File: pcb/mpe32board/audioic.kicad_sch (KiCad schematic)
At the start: 13 parts, among them J47 AudioJack3_Ground, U1 TAC5212IRGER

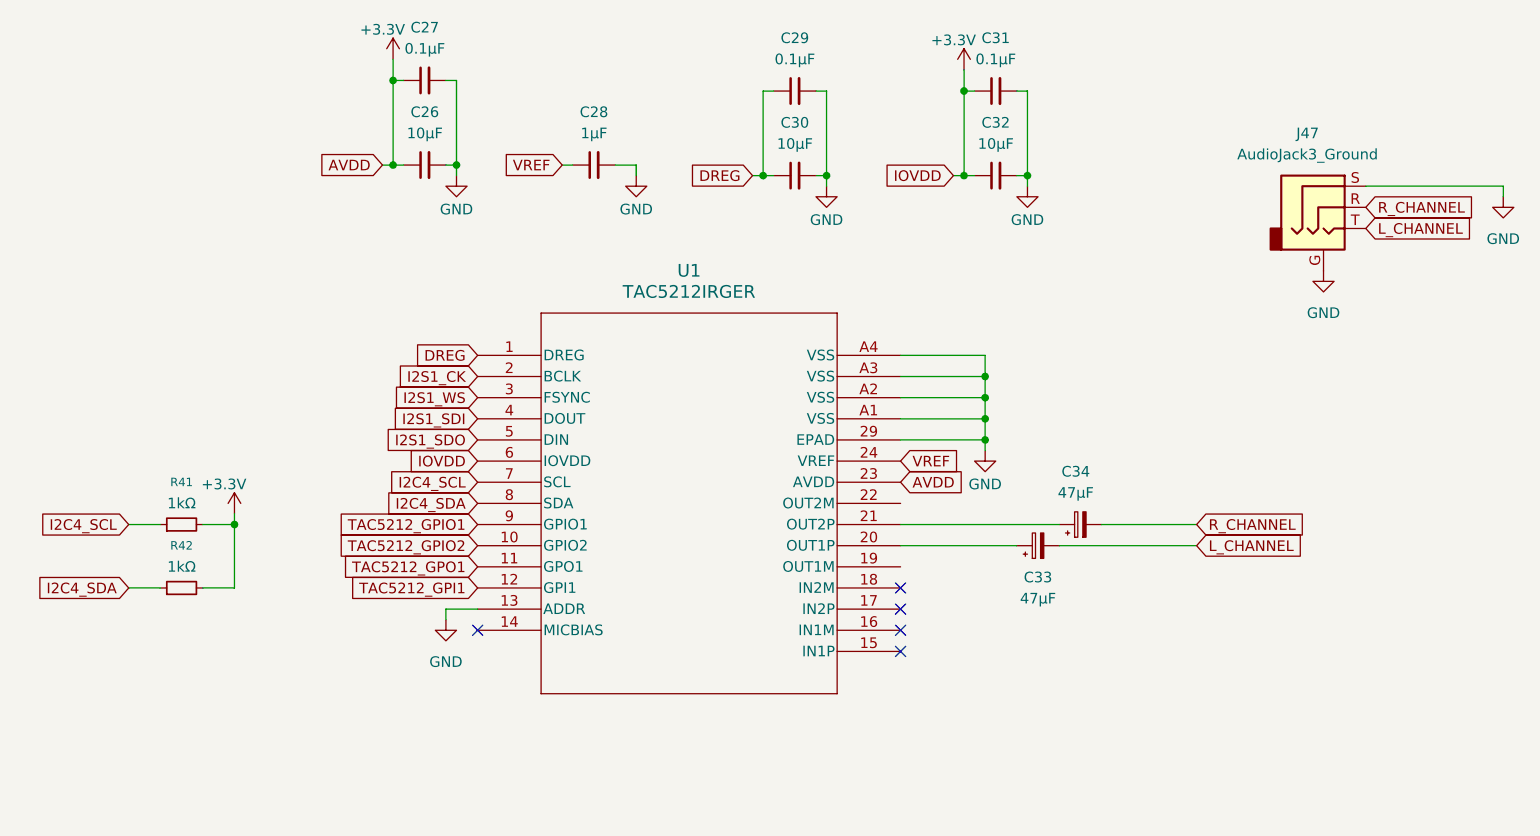
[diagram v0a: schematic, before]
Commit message: layout stuff
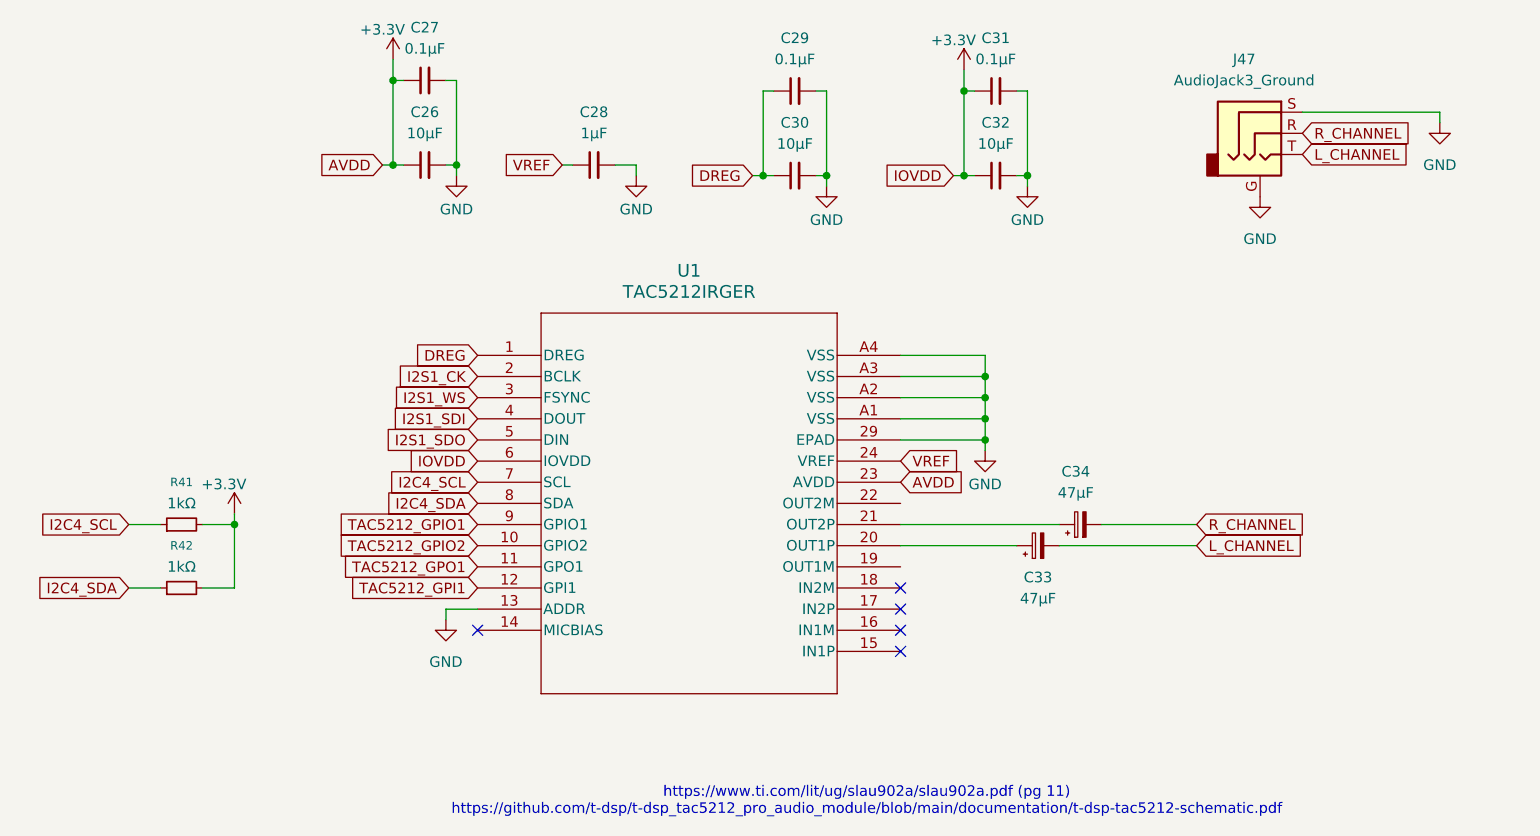
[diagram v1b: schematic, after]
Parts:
- C26, C27, C28, C29, C30, C31, C32, C33, C34: footprint (none) -> Capacitor_SMD:C_0603_1608Metric
- R41, R42: footprint (none) -> Resistor_SMD:R_0603_1608Metric
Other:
- note added: "https://www.ti.com/lit/ug/slau902a/slau902a.pdf (pg 11) https://github.com/t-dsp/t-dsp_tac5212_pro_audio_module/blob/main/documentation/t-dsp-tac5212-schematic.pdf"
- moved on the sheet: J47
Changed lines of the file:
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@@
 	(generator_version "9.0")
 	(paper "A4")
+	(text "https://www.ti.com/lit/ug/slau902a/slau902a.pdf (pg 11)\nhttps://github.com/t-dsp/t-dsp_tac5212_pro_audio_module/blob/main/documentation/t-dsp-tac5212-schematic.pdf"
+		(exclude_from_sim no)
+		(at 176.276 133.604 0)
+		(effects
+			(font
+				(size 1.27 1.27)
+			)
+		)
+	)
 	(junction
 		(at 119.38 57.15)
@@
 	(wire
 		(pts
-			(xy 252.73 60.96) (xy 252.73 59.69)
+			(xy 245.11 52.07) (xy 245.11 50.8)
 		)
 		(stroke
@@
 	(wire
 		(pts
-			(xy 252.73 59.69) (xy 236.22 59.69)
+			(xy 245.11 50.8) (xy 228.6 50.8)
 		)
 		(stroke
@@
 	(global_label "L_CHANNEL"
 		(shape input)
-		(at 236.22 64.77 0)
+		(at 228.6 55.88 0)
 		(fields_autoplaced yes)
 		(effects
@@
 		)
 		(property "Intersheetrefs" "${INTERSHEET_REFS}"
-			(at 249.7281 64.77 0)
+			(at 242.1081 55.88 0)
 			(effects
 				(font
@@
 	(global_label "R_CHANNEL"
 		(shape input)
-		(at 236.22 62.23 0)
+		(at 228.6 53.34 0)
 		(fields_autoplaced yes)
 		(effects
@@
 		)
 		(property "Intersheetrefs" "${INTERSHEET_REFS}"
-			(at 249.97 62.23 0)
+			(at 242.35 53.34 0)
 			(effects
 				(font
@@
 			)
 		)
-		(property "Footprint" ""
+		(property "Footprint" "Capacitor_SMD:C_0603_1608Metric"
 			(at 191.77 58.42 0)
 			(effects
@@
 			)
 		)
-		(property "Footprint" ""
+		(property "Footprint" "Capacitor_SMD:C_0603_1608Metric"
 			(at 167.64 48.26 0)
 			(effects
@@
 	(symbol
 		(lib_id "power:GND")
-		(at 231.14 69.85 0)
+		(at 223.52 60.96 0)
 		(unit 1)
 		(exclude_from_sim no)
@@
 		(fields_autoplaced yes)
 		(property "Reference" "#PWR0150"
-			(at 231.14 76.2 0)
+			(at 223.52 67.31 0)
 			(effects
 				(font
@@
 		)
 		(property "Value" "GND"
-			(at 231.14 74.93 0)
+			(at 223.52 66.04 0)
 			(effects
 				(font
@@
 		)
 		(property "Footprint" ""
-			(at 231.14 69.85 0)
+			(at 223.52 60.96 0)
 			(effects
 				(font
@@
 		)
 		(property "Datasheet" ""
-			(at 231.14 69.85 0)
+			(at 223.52 60.96 0)
 			(effects
 				(font
@@
 		)
 		(property "Description" "Power symbol creates a global label with name \"GND\" , ground"
-			(at 231.14 69.85 0)
+			(at 223.52 60.96 0)
 			(effects
 				(font
@@
 	(symbol
 		(lib_id "Connector_Audio:AudioJack3_Ground")
-		(at 231.14 62.23 0)
+		(at 223.52 53.34 0)
 		(unit 1)
 		(exclude_from_sim no)
@@
 		(fields_autoplaced yes)
 		(property "Reference" "J47"
-			(at 229.235 53.34 0)
+			(at 221.615 44.45 0)
 			(effects
 				(font
@@
 		)
 		(property "Value" "AudioJack3_Ground"
-			(at 229.235 55.88 0)
+			(at 221.615 46.99 0)
 			(effects
 				(font
@@
 		)
 		(property "Footprint" "Connector_Audio:Jack_3.5mm_CUI_SJ-3524-SMT_Horizontal"
-			(at 231.14 62.23 0)
+			(at 223.52 53.34 0)
 			(effects
 				(font
@@
 		)
 		(property "Datasheet" "~"
-			(at 231.14 62.23 0)
+			(at 223.52 53.34 0)
 			(effects
 				(font
@@
 		)
 		(property "Description" "Audio Jack, 3 Poles (Stereo / TRS), Grounded Sleeve"
-			(at 231.14 62.23 0)
+			(at 223.52 53.34 0)
 			(effects
 				(font
@@
 			)
 		)
-		(property "Footprint" ""
+		(property "Footprint" "Capacitor_SMD:C_0603_1608Metric"
 			(at 123.19 46.99 0)
 			(effects
@@
 			)
 		)
-		(property "Footprint" ""
+		(property "Footprint" "Capacitor_SMD:C_0603_1608Metric"
 			(at 143.51 57.15 0)
 			(effects
@@
 			)
 		)
-		(property "Footprint" ""
+		(property "Footprint" "Resistor_SMD:R_0603_1608Metric"
 			(at 93.98 107.95 0)
 			(effects
@@
 			)
 		)
-		(property "Footprint" ""
+		(property "Footprint" "Capacitor_SMD:C_0603_1608Metric"
 			(at 196.85 102.87 0)
 			(effects
@@
 	(symbol
 		(lib_id "power:GND")
-		(at 252.73 60.96 0)
+		(at 245.11 52.07 0)
 		(unit 1)
 		(exclude_from_sim no)
@@
 		(fields_autoplaced yes)
 		(property "Reference" "#PWR0159"
-			(at 252.73 67.31 0)
+			(at 245.11 58.42 0)
 			(effects
 				(font
@@
 		)
 		(property "Value" "GND"
-			(at 252.73 66.04 0)
+			(at 245.11 57.15 0)
 			(effects
 				(font
@@
 		)
 		(property "Footprint" ""
-			(at 252.73 60.96 0)
+			(at 245.11 52.07 0)
 			(effects
 				(font
@@
 		)
 		(property "Datasheet" ""
-			(at 252.73 60.96 0)
+			(at 245.11 52.07 0)
 			(effects
 				(font
@@
 		)
 		(property "Description" "Power symbol creates a global label with name \"GND\" , ground"
-			(at 252.73 60.96 0)
+			(at 245.11 52.07 0)
 			(effects
 				(font
@@
 			)
 		)
-		(property "Footprint" ""
+		(property "Footprint" "Capacitor_SMD:C_0603_1608Metric"
 			(at 167.64 58.42 0)
 			(effects
@@
 			)
 		)
-		(property "Footprint" ""
+		(property "Footprint" "Resistor_SMD:R_0603_1608Metric"
 			(at 93.98 100.33 0)
 			(effects
@@
 			)
 		)
-		(property "Footprint" ""
+		(property "Footprint" "Capacitor_SMD:C_0603_1608Metric"
 			(at 123.19 57.15 0)
 			(effects
@@
 			)
 		)
-		(property "Footprint" ""
+		(property "Footprint" "Capacitor_SMD:C_0603_1608Metric"
 			(at 201.93 100.33 0)
 			(effects
@@
 			)
 		)
-		(property "Footprint" ""
+		(property "Footprint" "Capacitor_SMD:C_0603_1608Metric"
 			(at 191.77 48.26 0)
 			(effects
